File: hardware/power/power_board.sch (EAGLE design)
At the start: 61 parts, among them IC1 LM321MF, IC2 LM321MF, J1 FASTON_MALE_RA_BLADE, J2 FASTON_MALE_RA_BLADE, J3 12v, J4 5v, J5 XT30PW-F, J6 XT30PW-F, J7 XT30PW-F, J8 XT30PW-F, U1 PDQ30-Q24-S5-D, U2 PDQ30-Q24-S12-D

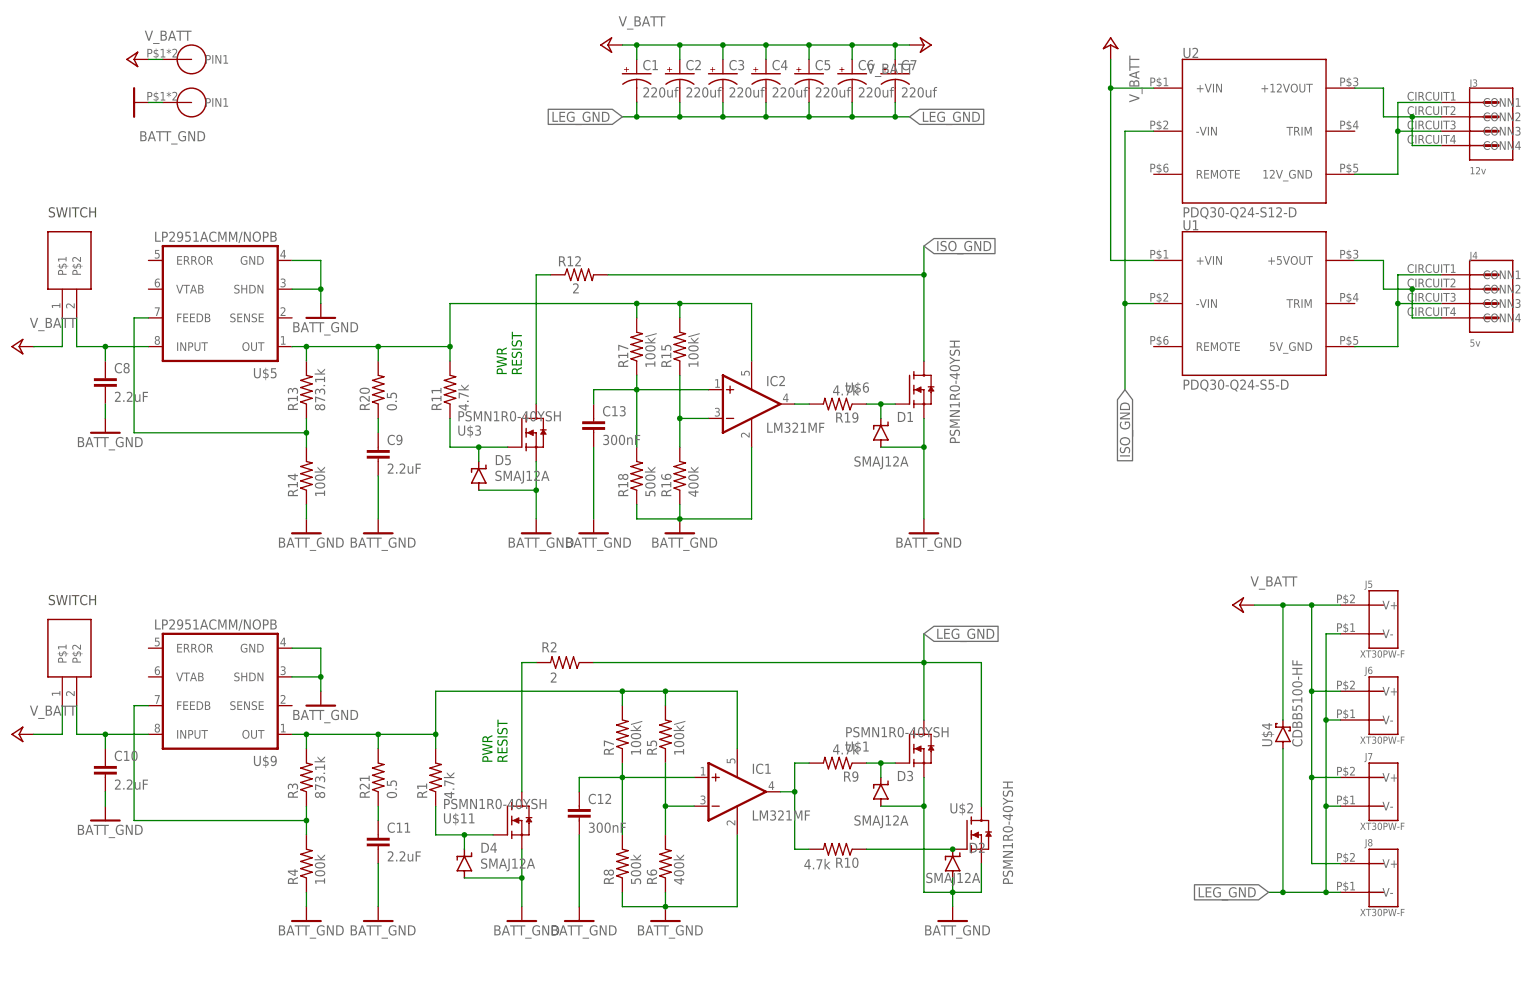
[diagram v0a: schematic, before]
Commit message: part moving
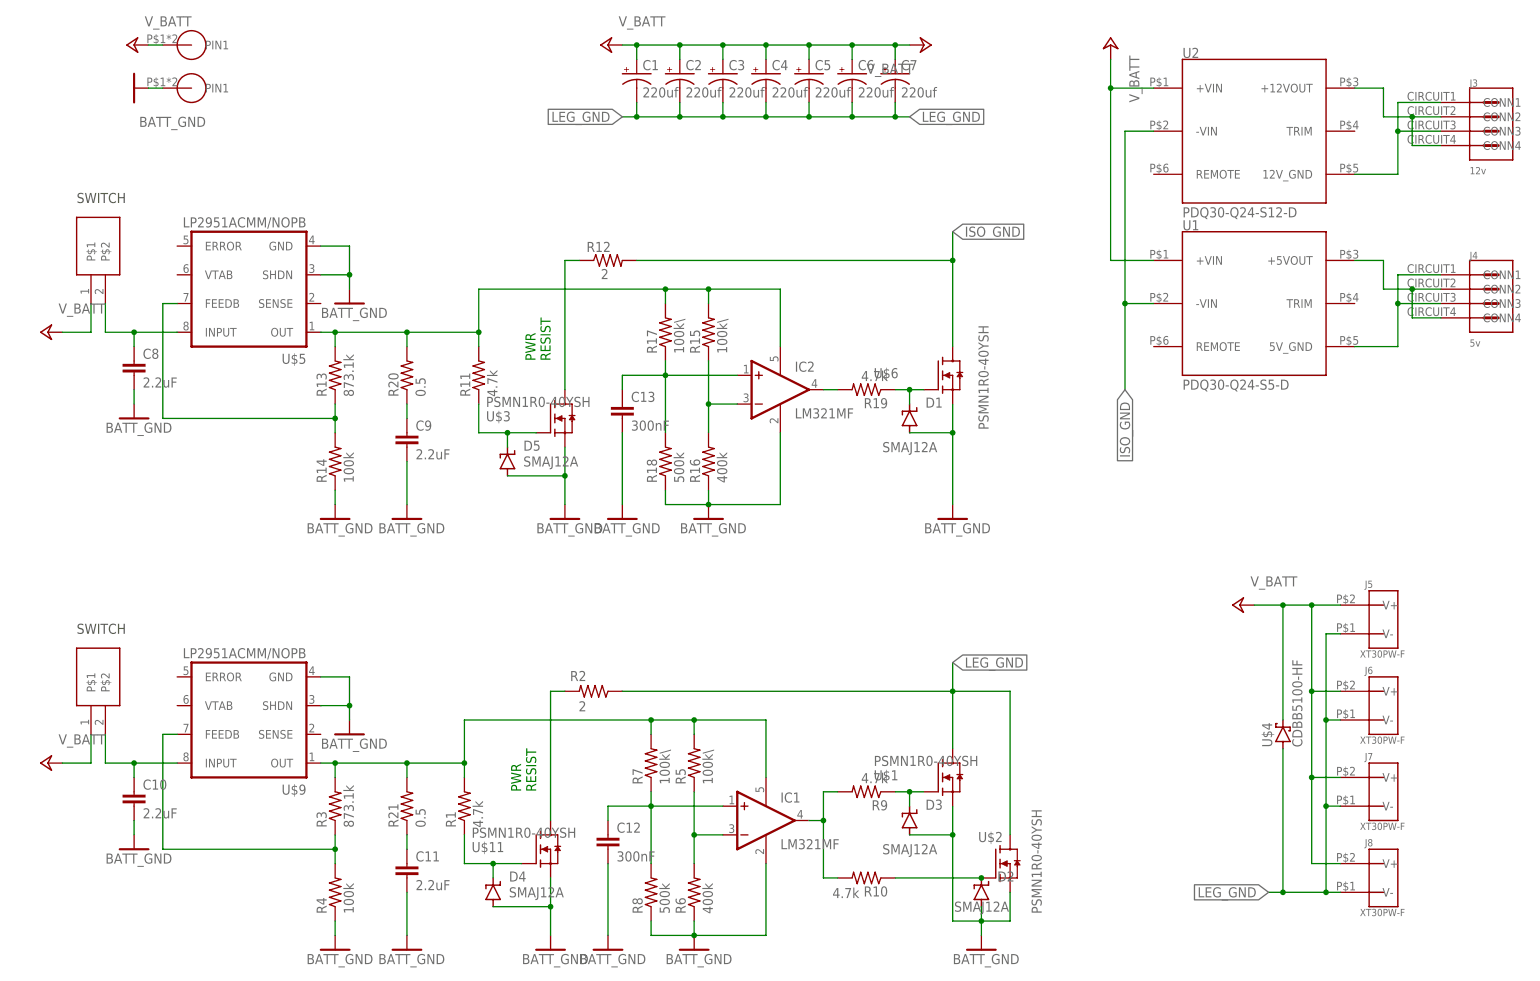
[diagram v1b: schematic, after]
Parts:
- C10, C11, C12, C13, C8, C9: device timlib:C0402 -> timlib:C_CERAMIC_0603
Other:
- moved on the sheet: C10, C11, C12, C13, C8, C9, D1, D2, D3, D4, D5, IC1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
